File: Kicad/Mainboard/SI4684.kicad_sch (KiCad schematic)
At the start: 96 parts, among them J1 Conn_01x03, J3 Headphones, J5 DISP LEFT, J6 DISP RIGHT, J7 Conn_01x02_Pin, J8 Conn_01x02_Pin, J9 Conn_01x02_Pin, Q2 2N7002, SW5 SW_Push, SW6 SW_Push, U1 MIC5504-1.8YM5, U12 SIQ-02FVS3, U14 SIQ-02FVS3, U2 BME680, U3 SI4684-A10-GM, U4 TCA9554PW, U5 TPA6130A2RTJTG4, U6 RT9013, X1 19.2MHz

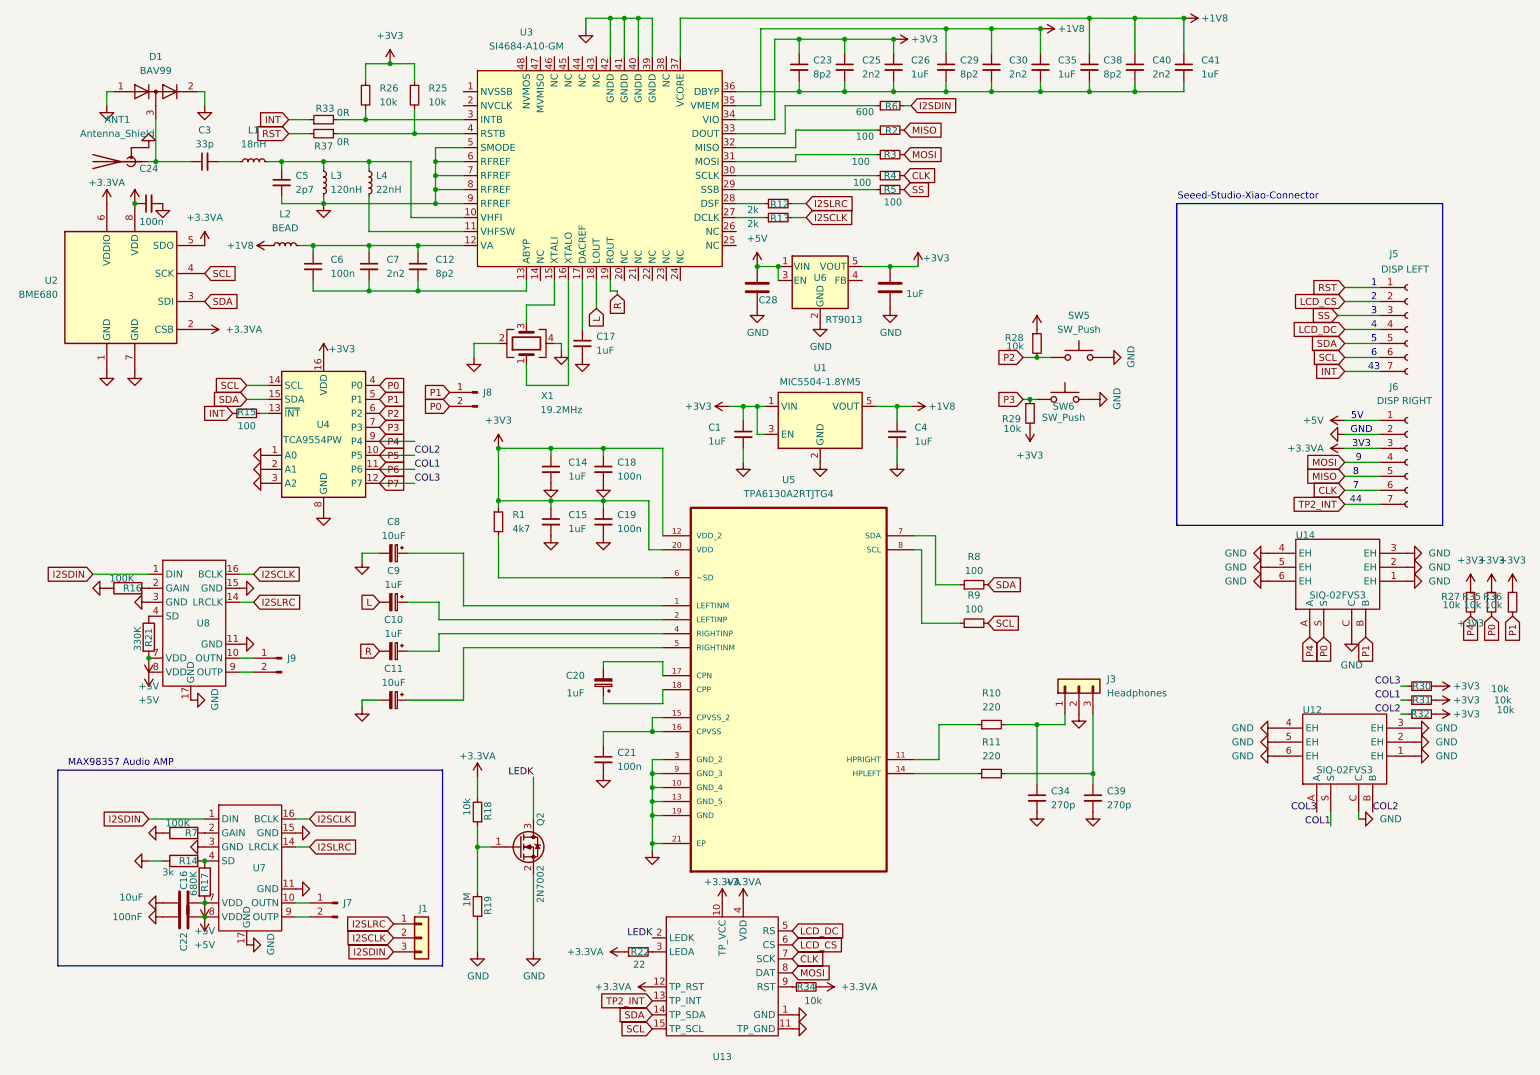
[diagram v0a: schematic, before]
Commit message: Add files via upload
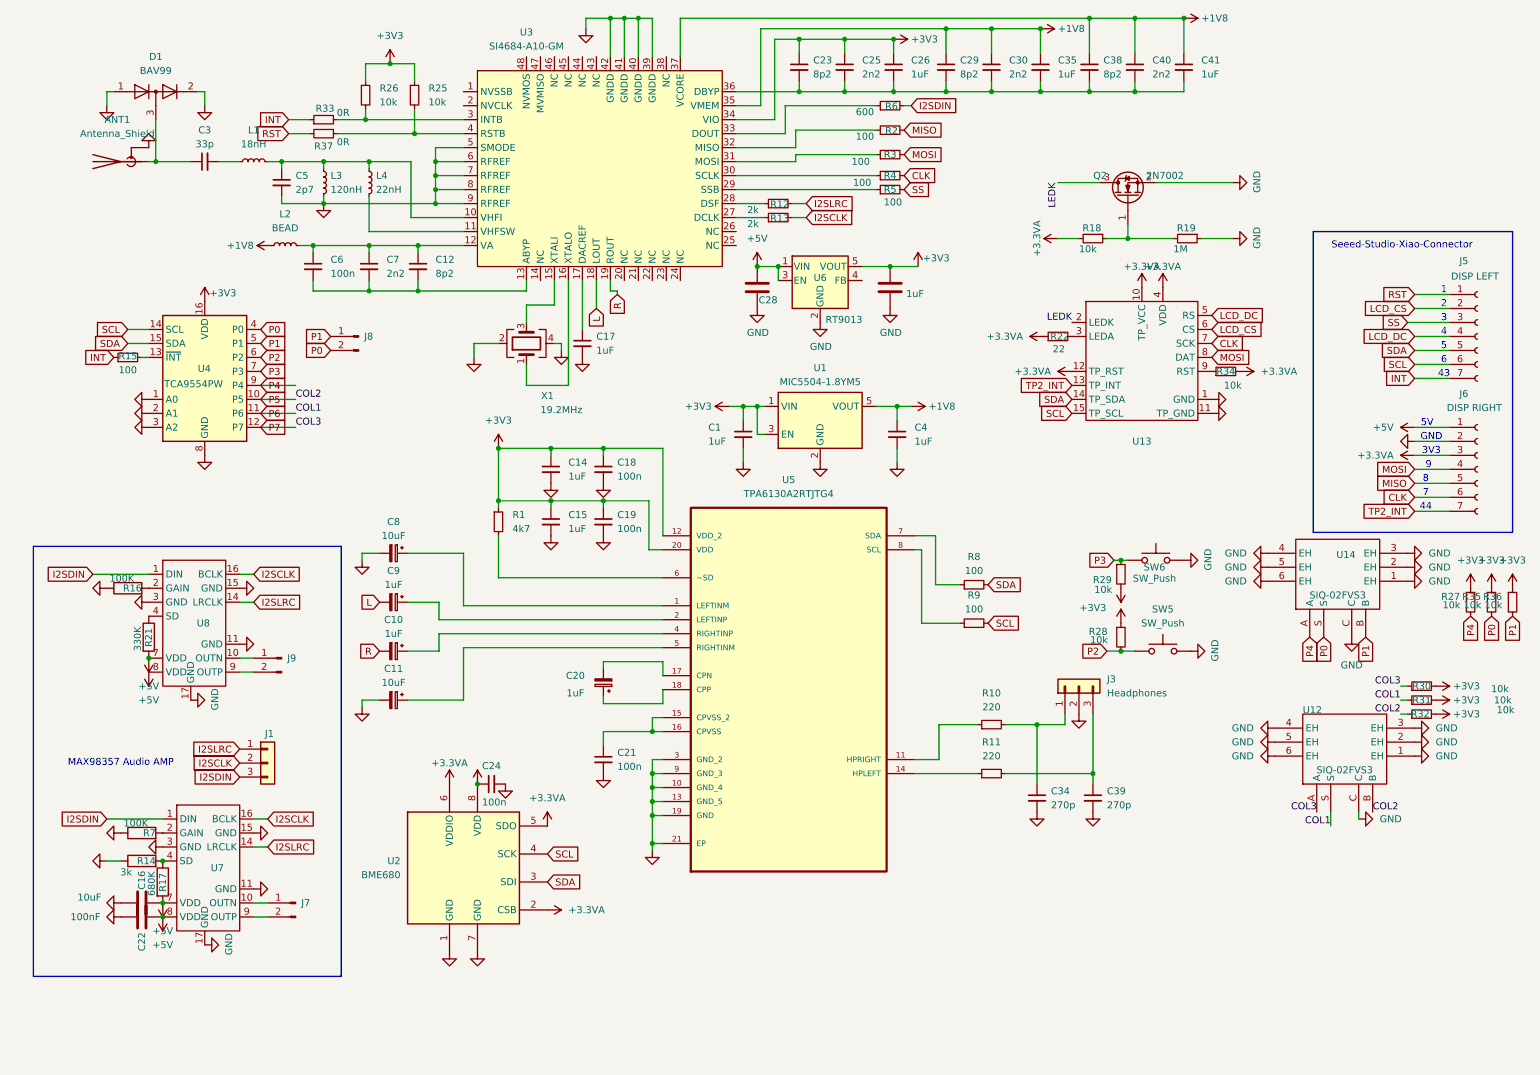
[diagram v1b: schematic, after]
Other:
- moved on the sheet: C16, C22, C24, J1, J5, J6, J7, J8, Q2, R14, R15, R17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
